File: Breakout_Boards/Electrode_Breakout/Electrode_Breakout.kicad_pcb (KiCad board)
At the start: 2 copper layers, 100 x 68 mm, 6 parts, among them J1 DB-9_Female, J2 DB-9_Female, J3 Conn_01x04_Pin, J4 Conn_01x04_Pin, J5 Conn_01x04_Pin, J7 Conn_01x03_Pin

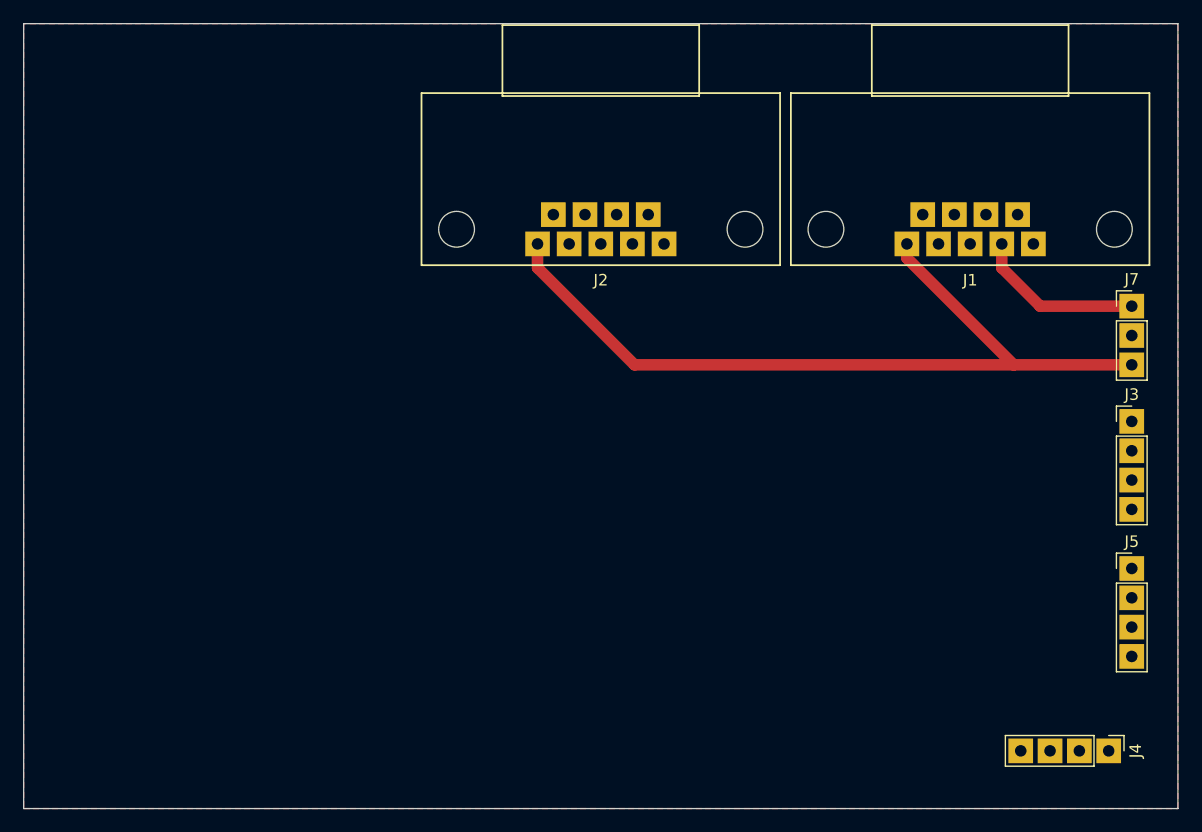
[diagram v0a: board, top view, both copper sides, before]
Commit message: Push Electrode_Breakout to Git
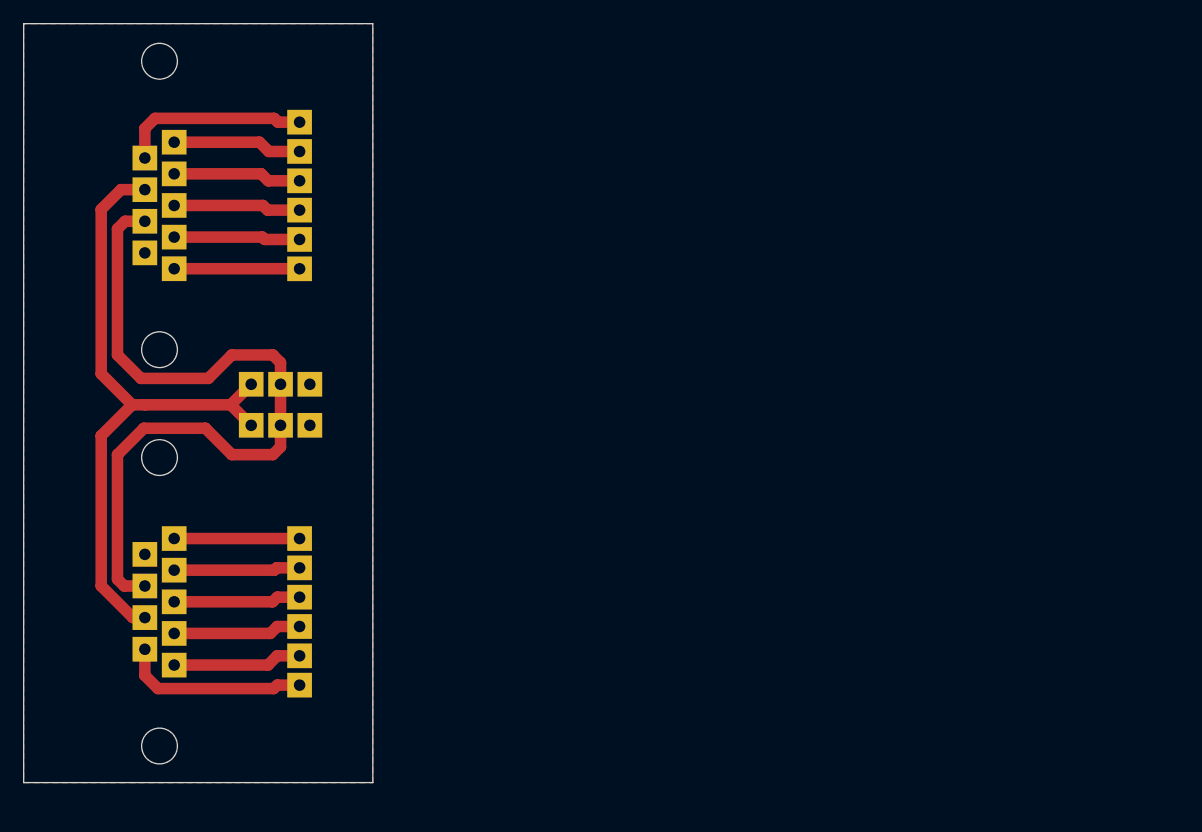
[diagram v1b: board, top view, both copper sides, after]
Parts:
- removed J7: Conn_01x03_Pin, Connector_PinHeader_2.54mm:PinHeader_1x03_P2.54mm_Vertical
- added J6: Conn_01x03, Connector_PinHeader_2.54mm:PinHeader_1x03_P2.54mm_Vertical, B.Cu at (24.8, 31.2)
- J1, J2: moved to B.Cu
- J3, J4: value Conn_01x04_Pin -> Conn_01x06; footprint Connector_PinHeader_2.54mm:PinHeader_1x04_P2.54mm_Vertical -> Connector_PinHeader_2.54mm:PinHeader_1x06_P2.54mm_Vertical; moved to B.Cu
- J5: value Conn_01x04_Pin -> Conn_01x03; footprint Connector_PinHeader_2.54mm:PinHeader_1x04_P2.54mm_Vertical -> Connector_PinHeader_2.54mm:PinHeader_1x03_P2.54mm_Vertical; moved to B.Cu
- moved J1 82.5 mm to (0.10, 15.8), turned to -90 degrees
- moved J3 76.6 mm to (23.9, 8.53), turned to 180 degrees
- moved J4 72.5 mm to (23.9, 44.6), turned to 180 degrees
- moved J5 72.3 mm to (24.8, 34.8), turned to 90 degrees
- moved J2 66.5 mm to (0.10, 50.1), turned to -90 degrees
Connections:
- J1 pad 1: /ADC1 -> /CUR1
- J1 pad 2: /+12V -> /CUR2
- J1 pad 3: /CUR1 -> /SEL1
- J1 pad 4: /SEL1 -> /SEL2
- J1 pad 5: /-12V -> /ADC2
- J1 pad 7: /CUR2 -> /-12V
- J1 pad 8: /SEL2 -> /+12V
- J1 pad 9: /ADC2 -> /ADC1
- J2 pad 2: /+12V -> /CUR3
- J2 pad 3: /CUR3 -> /CUR4
- J2 pad 5: /-12V -> /SEL4
- J2 pad 6: GND -> /ADC4
- J2 pad 7: /CUR4 -> /+12V
- J2 pad 8: /SEL4 -> /-12V
- J2 pad 9: /ADC4 -> GND
- J3 pad 3: /ADC3 -> /SEL2
- J3 pad 4: /ADC4 -> /SEL1
- J4 pad 1: /SEL1 -> /SEL4
- J4 pad 2: /SEL2 -> /SEL3
- J4 pad 3: /SEL3 -> /CUR4
- J4 pad 4: /SEL4 -> /CUR3
- J5 pad 1: /CUR1 -> GND
- J5 pad 2: /CUR2 -> /-12V
- J5 pad 3: /CUR3 -> /+12V
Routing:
- net /+12V: track 14.7 -> 57.8 mm
- net /ADC1: track 0.00 -> 16.5 mm
- net /ADC4: track 0.00 -> 16.3 mm
- net /ADC2: track 0.00 -> 11.2 mm
- net /ADC3: track 0.00 -> 11.2 mm
- net /SEL2: track 0.00 -> 11.1 mm
- net /CUR3: track 0.00 -> 11.1 mm
- net /SEL1: track 0.00 -> 11.0 mm
- net /CUR4: track 0.00 -> 11.0 mm
- net /CUR2: track 0.00 -> 11.0 mm
- net /SEL3: track 0.00 -> 10.9 mm
- net /CUR1: track 0.00 -> 10.9 mm
- net /SEL4: track 0.00 -> 10.9 mm
- net /-12V: track 71.3 -> 66.7 mm
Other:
- board size 100 x 68 mm -> 30.2 x 65.8 mm
